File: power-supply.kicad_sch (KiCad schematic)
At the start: 25 parts, among them Q10 AO3401A, Q9 AO3401A, U8 TPS61230DRC, U9 LM3670MF

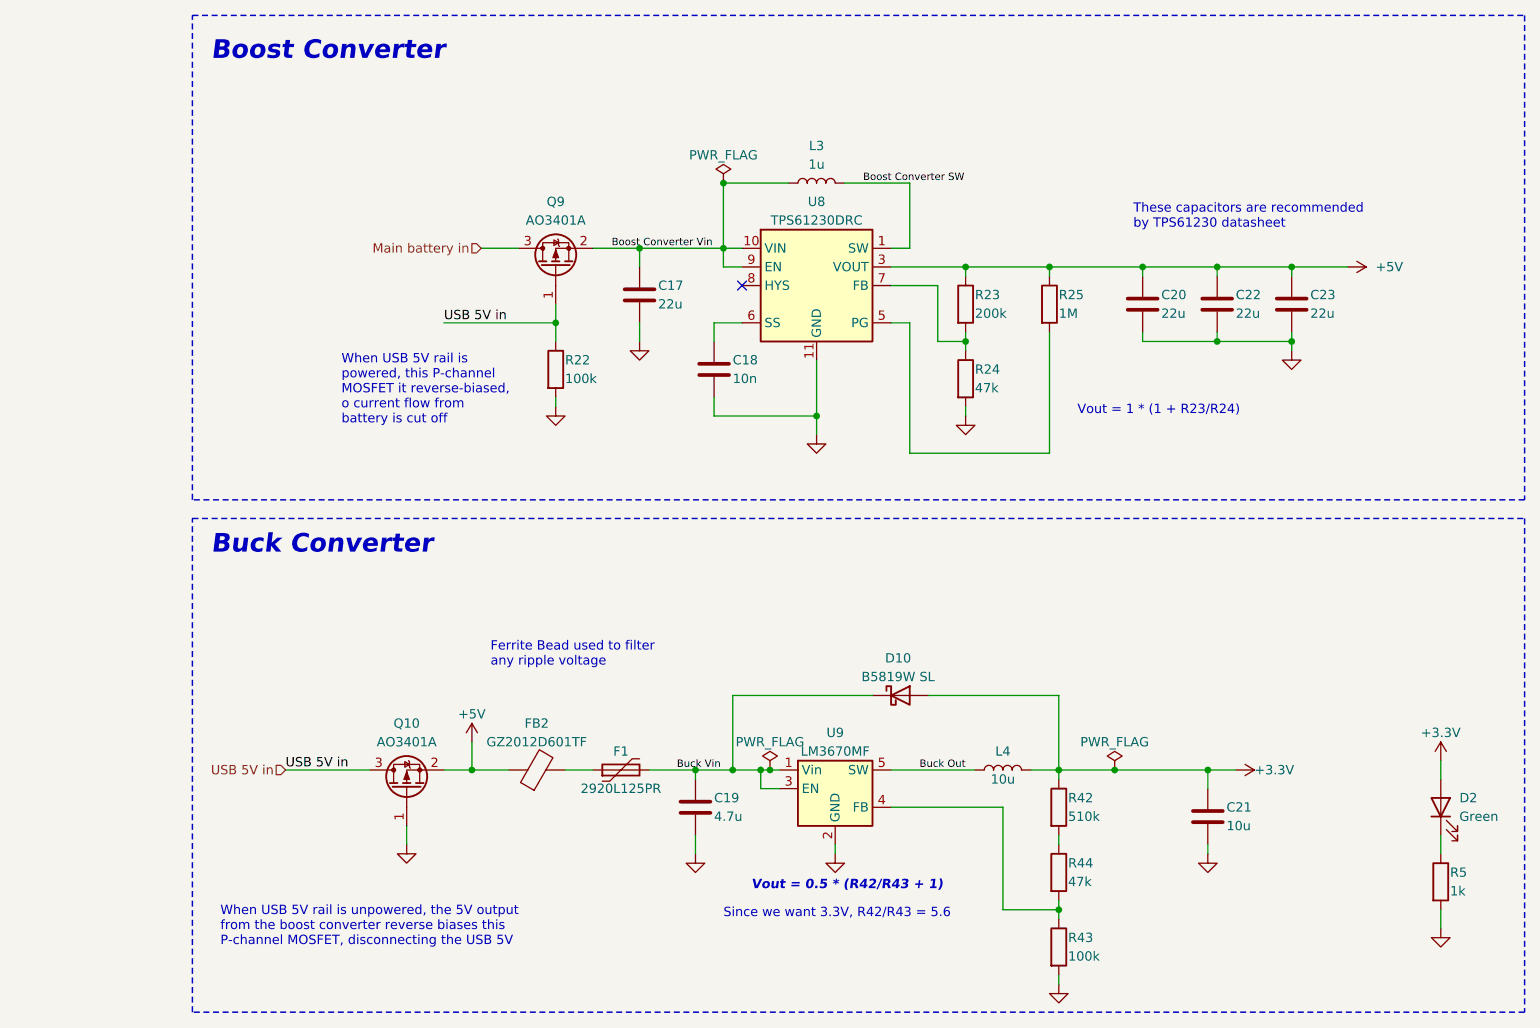
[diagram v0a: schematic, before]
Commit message: Added new buck converter
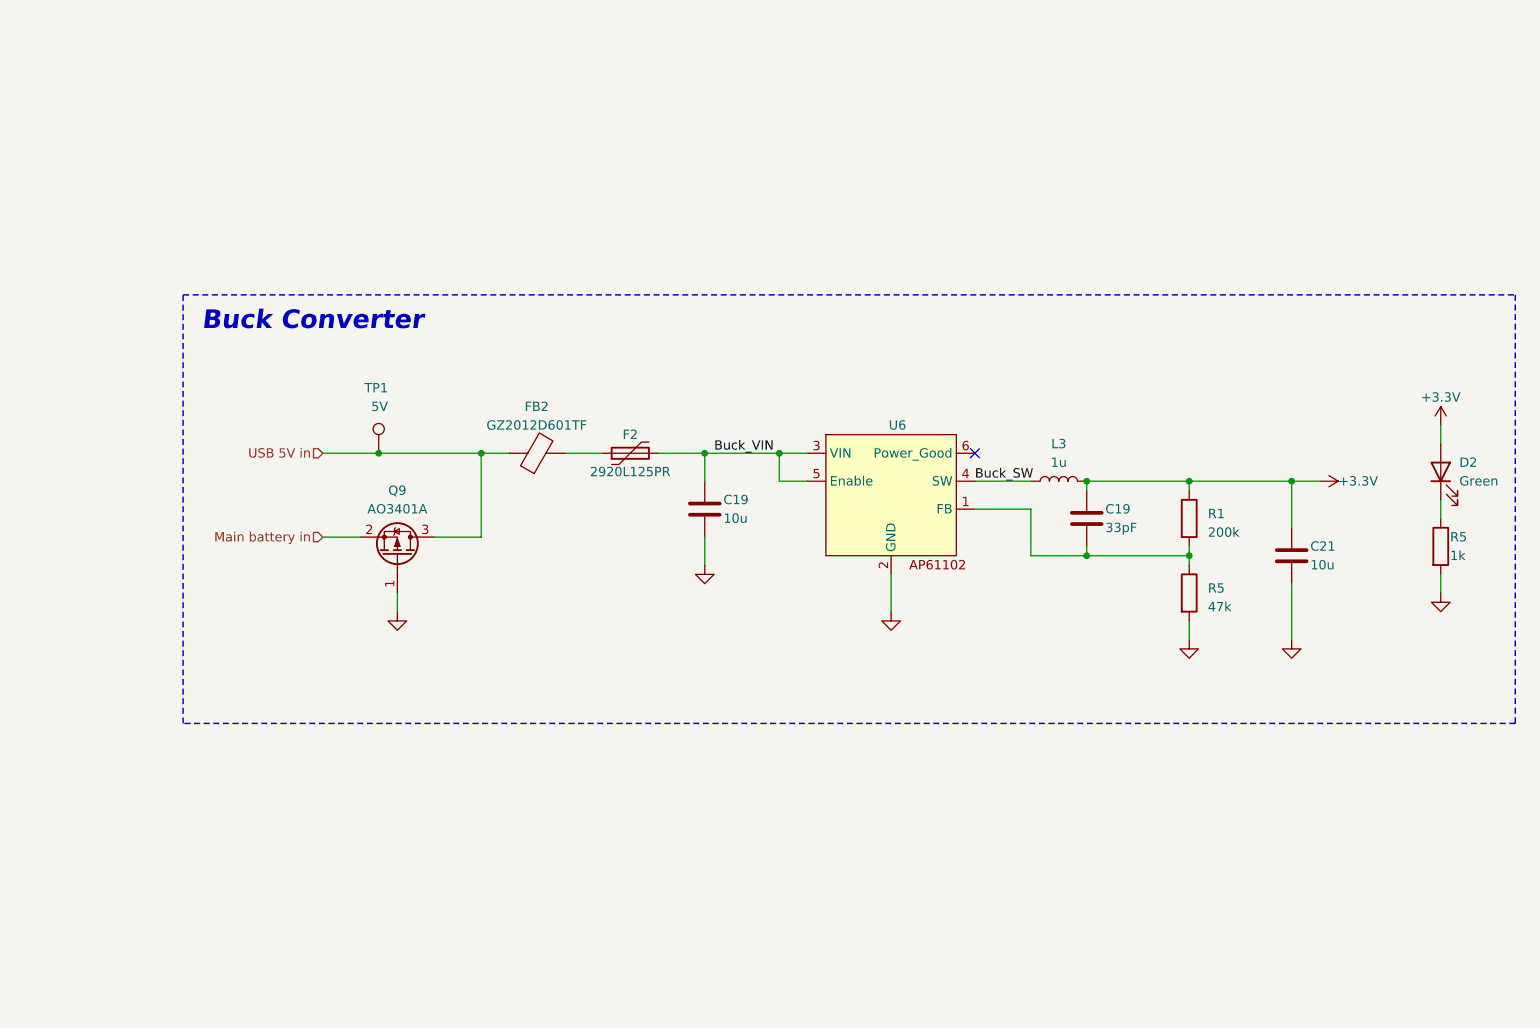
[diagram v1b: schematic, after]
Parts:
- removed C17, C20, C22, C23: 22u, Capacitor_SMD:C_0805_2012Metric, symbol Device:C
- removed C18: 10n, Capacitor_SMD:C_0402_1005Metric, symbol Device:C
- removed C19: 4.7u, Capacitor_SMD:C_0603_1608Metric, symbol Device:C
- removed D10: B5819W SL, Diode_SMD:D_SOD-123, symbol Device:D_Schottky
- removed F1: 2920L125PR, Fuse:Fuse_0805_2012Metric, symbol Device:Polyfuse
- removed L4: 10u, Inductor_SMD:L_Sunlord_SWPA4030S, symbol Device:L
- removed Q10: AO3401A, Package_TO_SOT_SMD:SOT-23, symbol Transistor_FET:AO3401A
- removed R22, R43: 100k, Resistor_SMD:R_0402_1005Metric, symbol Device:R
- removed R23: 200k, Resistor_SMD:R_0402_1005Metric, symbol Device:R
- removed R24, R44: 47k, Resistor_SMD:R_0402_1005Metric, symbol Device:R
- removed R25: 1M, Resistor_SMD:R_0402_1005Metric, symbol Device:R
- removed R42: 510k, Resistor_SMD:R_0603_1608Metric, symbol Device:R
- removed U8: TPS61230DRC, Package_SON:Texas_S-PVSON-N10_ThermalVias, symbol Regulator_Switching:TPS61230DRC
- removed U9: LM3670MF, Package_TO_SOT_SMD:TSOT-23-5, symbol Regulator_Switching:LM3670MF
- added C19: 33pF, Capacitor_SMD:C_0402_1005Metric, symbol Device:C
- added C19: 10u, Capacitor_SMD:C_0603_1608Metric, symbol Device:C
- added F2: 2920L125PR, Fuse:Fuse_0805_2012Metric, symbol Device:Polyfuse
- added R1: 200k, Resistor_SMD:R_0402_1005Metric, symbol Device:R
- added R5: 47k, Resistor_SMD:R_0402_1005Metric, symbol Device:R
- added TP1: 5V, TestPoint:TestPoint_Pad_D1.5mm, symbol Connector:TestPoint
- added U6: ~, Package_TO_SOT_SMD:SOT-563, symbol custom-symbols:AP61102
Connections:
- net +5V is gone; now on net USB 5V in: FB2.1
- net Boost Converter SW is gone; now on net +3.3V: L3.2
- net +3.3V: now also C19.1, R1.1
- net GND: now also Q9.1 (G), C19.2, R5.2, U6.2 (GND)
- net Main battery in: now also Q9.2 (S); no longer Q9.3 (D)
- net USB 5V in: now also Q9.3 (D), TP1.1; no longer Q9.1 (G)
- net at FB2.2: now also F2.1
- net Boost Converter Vin renamed Buck_SW
- net Buck_SW: now also U6.4 (SW); no longer Q9.2 (S)
- new net: C19.2, R1.2, R5.1, U6.1 (FB)
- new net Buck_VIN: C19.1, F2.2, U6.3 (VIN), U6.5 (Enable)
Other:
- note removed: "Boost Converter"
- note removed: "Ferrite Bead used to filter any ripple voltage"
- note removed: "Since we want 3.3V, R42/R43 = 5.6"
- note removed: "These capacitors are recommended by TPS61230 datasheet"
- note removed: "Vout = 0.5 * (R42/R43 + 1)"
- note removed: "Vout = 1 * (1 + R23/R24)"
- note removed: "When USB 5V rail is powered, this P-channel MOSFET it reverse-biased, o current flow from battery is cut off"
- note removed: "When USB 5V rail is unpowered, the 5V output from the boost converter reverse biases this P-channel MOSFET, disconnecting the USB 5V"
- moved on the sheet: D2, Q9, R5

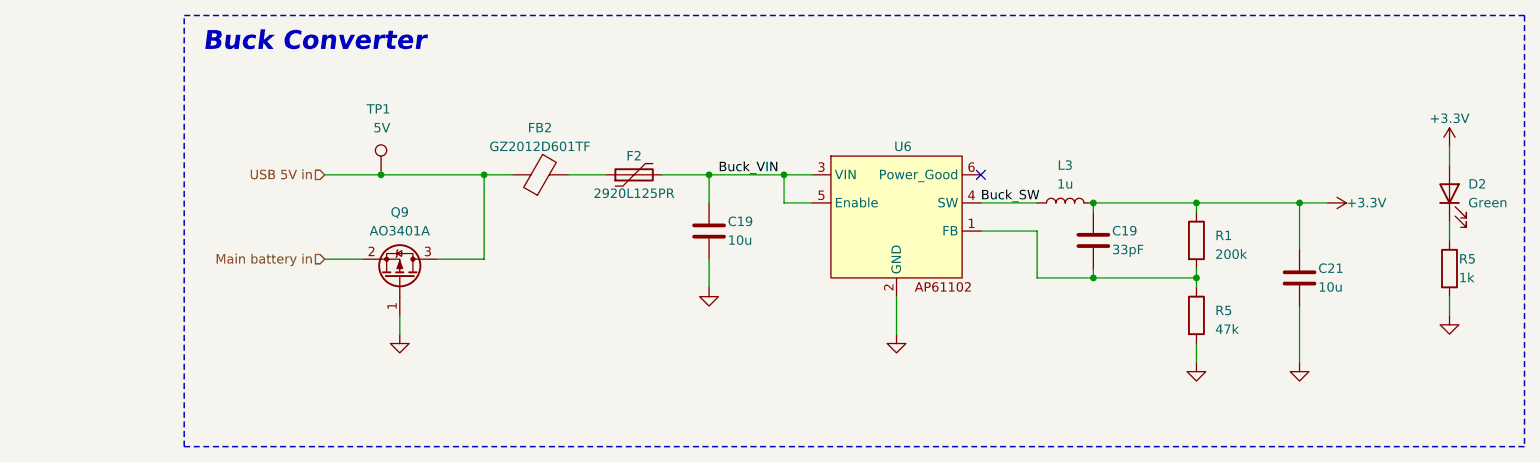
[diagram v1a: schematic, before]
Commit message: added switch to USB power and to bypass screw switch for main battery
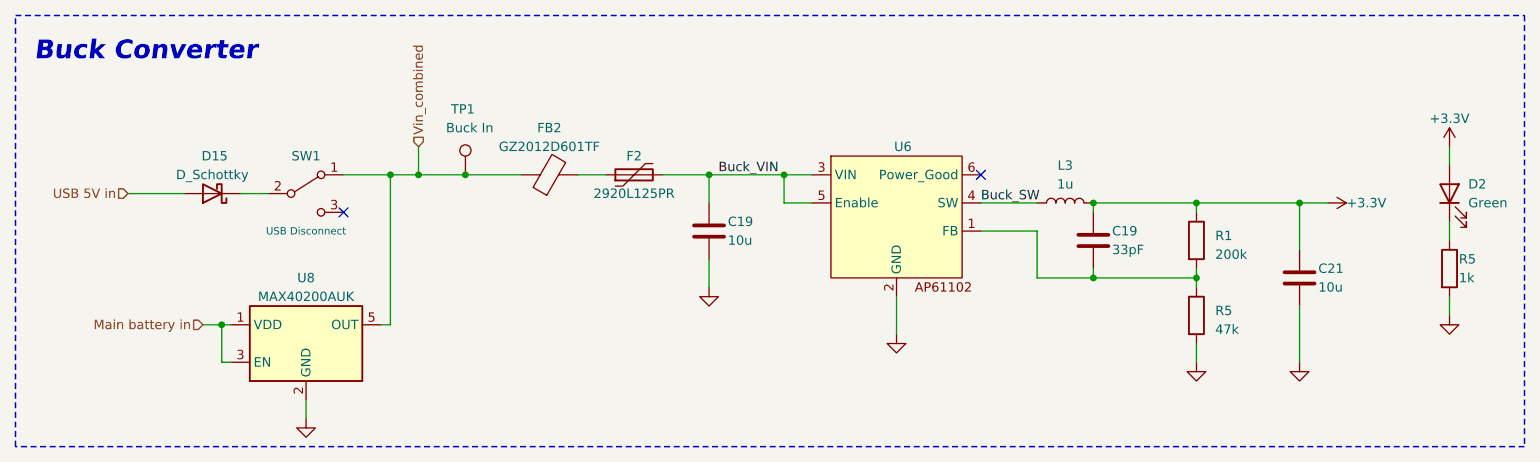
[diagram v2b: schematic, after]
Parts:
- removed Q9: AO3401A, Package_TO_SOT_SMD:SOT-23, symbol Transistor_FET:AO3401A
- added D15: D_Schottky, Diode_SMD:D_SOD-323, symbol Device:D_Schottky
- added SW1: USB Disconnect, Button_Switch_SMD:SW_SPDT_PCM12, symbol Switch:SW_SPDT
- added U8: MAX40200AUK, Package_TO_SOT_SMD:SOT-23-5, symbol Analog_Switch:MAX40200AUK
- TP1: value 5V -> Buck In
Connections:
- net GND: now also U8.2 (GND)
- net Main battery in: now also U8.1 (VDD), U8.3 (EN)
- net USB 5V in: now also D15.2 (A); no longer FB2.1, TP1.1
- new net: D15.1 (K), SW1.2 (B)
- new net Vin_combined: FB2.1, SW1.1 (A), TP1.1, U8.5 (OUT)
- no-connect marks 1 -> 2
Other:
- moved on the sheet: FB2, TP1

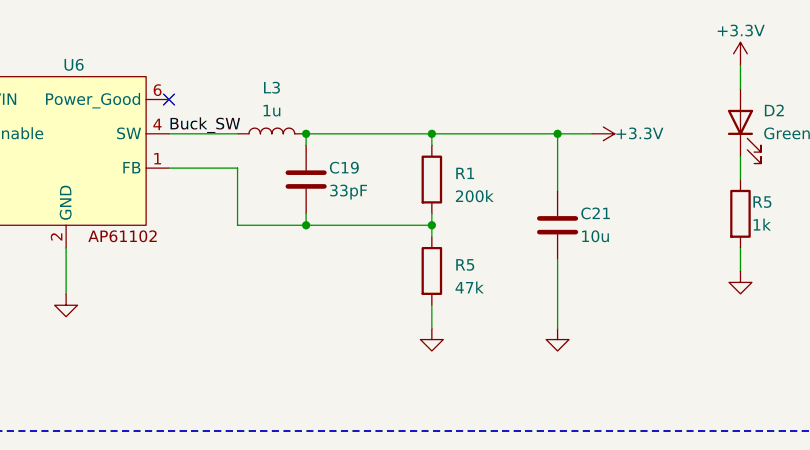
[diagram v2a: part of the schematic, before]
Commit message: Changed Vreg to 3.3 volts from 3.15
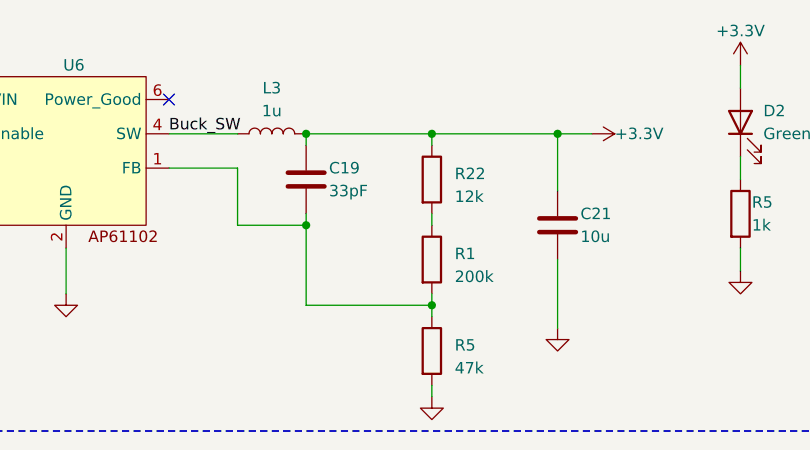
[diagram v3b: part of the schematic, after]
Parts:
- added R22: 12k, Resistor_SMD:R_0402_1005Metric, symbol Device:R
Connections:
- net +3.3V: now also R22.1; no longer R1.1
- new net: R1.1, R22.2
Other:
- moved on the sheet: R1, R5
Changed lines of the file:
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@@
   (junction (at 180.34 99.06) (diameter 0) (color 0 0 0 0)
   )
+  (junction (at 194.31 107.95) (diameter 0) (color 0 0 0 0)
+  )
   (junction (at 62.23 105.41) (diameter 0) (color 0 0 0 0)
   )
@@
   )
   (junction (at 128.27 85.09) (diameter 0) (color 0 0 0 0)
-  )
-  (junction (at 194.31 99.06) (diameter 0) (color 0 0 0 0)
   )
   (junction (at 180.34 88.9) (diameter 0) (color 0 0 0 0)
@@
   (no_connect (at 78.74 90.17))
   (no_connect (at 165.1 85.09))
+  (wire (pts (xy 194.31 107.95) (xy 194.31 109.22))
+    (stroke (width 0) (type default))
+  )
   (wire (pts (xy 78.74 85.09) (xy 85.09 85.09))
     (stroke (width 0) (type default))
@@
     (stroke (width 0) (type default))
   )
-  (wire (pts (xy 180.34 99.06) (xy 194.31 99.06))
+  (wire (pts (xy 180.34 107.95) (xy 194.31 107.95))
     (stroke (width 0) (type default))
   )
@@
     (stroke (width 0) (type default))
   )
-  (wire (pts (xy 194.31 107.95) (xy 194.31 110.49))
+  (wire (pts (xy 194.31 116.84) (xy 194.31 118.11))
     (stroke (width 0) (type default))
   )
@@
     (stroke (width 0) (type default))
   )
+  (wire (pts (xy 194.31 99.06) (xy 194.31 97.79))
+    (stroke (width 0) (type default))
+  )
+  (wire (pts (xy 180.34 107.95) (xy 180.34 99.06))
+    (stroke (width 0) (type default))
+  )
   (wire (pts (xy 110.49 85.09) (xy 114.3 85.09))
     (stroke (width 0) (type default))
@@
     (stroke (width 0) (type default))
   )
-  (wire (pts (xy 194.31 99.06) (xy 194.31 100.33))
+  (wire (pts (xy 194.31 106.68) (xy 194.31 107.95))
     (stroke (width 0) (type default))
   )
@@
   )
   (wire (pts (xy 95.25 85.09) (xy 102.87 85.09))
-    (stroke (width 0) (type default))
-  )
-  (wire (pts (xy 194.31 97.79) (xy 194.31 99.06))
     (stroke (width 0) (type default))
   )
@@
     )
   )
+  (symbol (lib_id "Device:R") (at 194.31 93.98 0) (unit 1)
+    (in_bom yes) (on_board yes) (dnp no) (fields_autoplaced)
+    (property "Reference" "R22" (at 196.85 93.345 0)
+      (effects (font (size 1.27 1.27)) (justify left))
+    )
+    (property "Value" "12k" (at 196.85 95.885 0)
+      (effects (font (size 1.27 1.27)) (justify left))
+    )
+    (property "Footprint" "Resistor_SMD:R_0402_1005Metric" (at 192.532 93.98 90)
+      (effects (font (size 1.27 1.27)) hide)
+    )
+    (property "Datasheet" "~" (at 194.31 93.98 0)
+      (effects (font (size 1.27 1.27)) hide)
+    )
+    (pin "1")
+    (pin "2")
+    (instances
+      (project "Flight Computer"
+        (path "/0c1188a1-706b-46cd-a73a-5b3f8187d77a/afc466af-6d84-4e19-b5b5-aea43618ea20/d3a2bed6-f277-4c18-9b19-db934fe0c906"
+          (reference "R22") (unit 1)
+        )
+      )
+    )
+  )
   (symbol (lib_id "Device:R") (at 228.6 97.79 0) (unit 1)
     (in_bom yes) (on_board yes) (dnp no)
@@
     )
   )
-  (symbol (lib_id "Device:R") (at 194.31 93.98 0) (unit 1)
-    (in_bom yes) (on_board yes) (dnp no) (fields_autoplaced)
-    (property "Reference" "R1" (at 196.85 93.345 0)
-      (effects (font (size 1.27 1.27)) (justify left))
-    )
-    (property "Value" "200k" (at 196.85 95.885 0)
-      (effects (font (size 1.27 1.27)) (justify left))
-    )
-    (property "Footprint" "Resistor_SMD:R_0402_1005Metric" (at 192.532 93.98 90)
-      (effects (font (size 1.27 1.27)) hide)
-    )
-    (property "Datasheet" "~" (at 194.31 93.98 0)
+  (symbol (lib_id "Device:R") (at 194.31 102.87 0) (unit 1)
+    (in_bom yes) (on_board yes) (dnp no) (fields_autoplaced)
+    (property "Reference" "R1" (at 196.85 102.235 0)
+      (effects (font (size 1.27 1.27)) (justify left))
+    )
+    (property "Value" "200k" (at 196.85 104.775 0)
+      (effects (font (size 1.27 1.27)) (justify left))
+    )
+    (property "Footprint" "Resistor_SMD:R_0402_1005Metric" (at 192.532 102.87 90)
+      (effects (font (size 1.27 1.27)) hide)
+    )
+    (property "Datasheet" "~" (at 194.31 102.87 0)
       (effects (font (size 1.27 1.27)) hide)
     )
@@
     )
   )
-  (symbol (lib_id "Device:R") (at 194.31 104.14 0) (unit 1)
-    (in_bom yes) (on_board yes) (dnp no) (fields_autoplaced)
-    (property "Reference" "R5" (at 196.85 103.505 0)
-      (effects (font (size 1.27 1.27)) (justify left))
-    )
-    (property "Value" "47k" (at 196.85 106.045 0)
-      (effects (font (size 1.27 1.27)) (justify left))
-    )
-    (property "Footprint" "Resistor_SMD:R_0402_1005Metric" (at 192.532 104.14 90)
-      (effects (font (size 1.27 1.27)) hide)
-    )
-    (property "Datasheet" "~" (at 194.31 104.14 0)
+  (symbol (lib_id "Device:R") (at 194.31 113.03 0) (unit 1)
+    (in_bom yes) (on_board yes) (dnp no) (fields_autoplaced)
+    (property "Reference" "R5" (at 196.85 112.395 0)
+      (effects (font (size 1.27 1.27)) (justify left))
+    )
+    (property "Value" "47k" (at 196.85 114.935 0)
+      (effects (font (size 1.27 1.27)) (justify left))
+    )
+    (property "Footprint" "Resistor_SMD:R_0402_1005Metric" (at 192.532 113.03 90)
+      (effects (font (size 1.27 1.27)) hide)
+    )
+    (property "Datasheet" "~" (at 194.31 113.03 0)
       (effects (font (size 1.27 1.27)) hide)
     )
@@
     )
   )
-  (symbol (lib_id "power:GND") (at 194.31 110.49 0) (unit 1)
-    (in_bom yes) (on_board yes) (dnp no) (fields_autoplaced)
-    (property "Reference" "#PWR061" (at 194.31 116.84 0)
-      (effects (font (size 1.27 1.27)) hide)
-    )
-    (property "Value" "GND" (at 194.31 115.57 0)
-      (effects (font (size 1.27 1.27)) hide)
-    )
-    (property "Footprint" "" (at 194.31 110.49 0)
-      (effects (font (size 1.27 1.27)) hide)
-    )
-    (property "Datasheet" "" (at 194.31 110.49 0)
-      (effects (font (size 1.27 1.27)) hide)
-    )
+  (symbol (lib_id "power:GND") (at 194.31 118.11 0) (unit 1)
+    (in_bom yes) (on_board yes) (dnp no) (fields_autoplaced)
+    (property "Reference" "#PWR061" (at 194.31 124.46 0)
+      (effects (font (size 1.27 1.27)) hide)
+    )
+    (property "Value" "GND" (at 194.31 123.19 0)
+      (effects (font (size 1.27 1.27)) hide)
+    )
+    (property "Footprint" "" (at 194.31 118.11 0)
+      (effects (font (size 1.27 1.27)) hide)
+    )
+    (property "Datasheet" "" (at 194.31 118.11 0)
+      (effects (font (size 1.27 1.27)) hide)
+    )
